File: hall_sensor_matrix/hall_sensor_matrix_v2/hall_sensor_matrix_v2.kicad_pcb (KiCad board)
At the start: 2 copper layers, 60 parts, among them J1 CTRL, J2 COL, J3 ROW, Q1 VP3203, Q2 VP3203, Q3 VP3203, Q4 VP3203, Q5 VP3203, Q6 VP3203, Q7 VP3203, Q8 VP3203, U1 74LS595, U2 74LS597, U3 74LS597

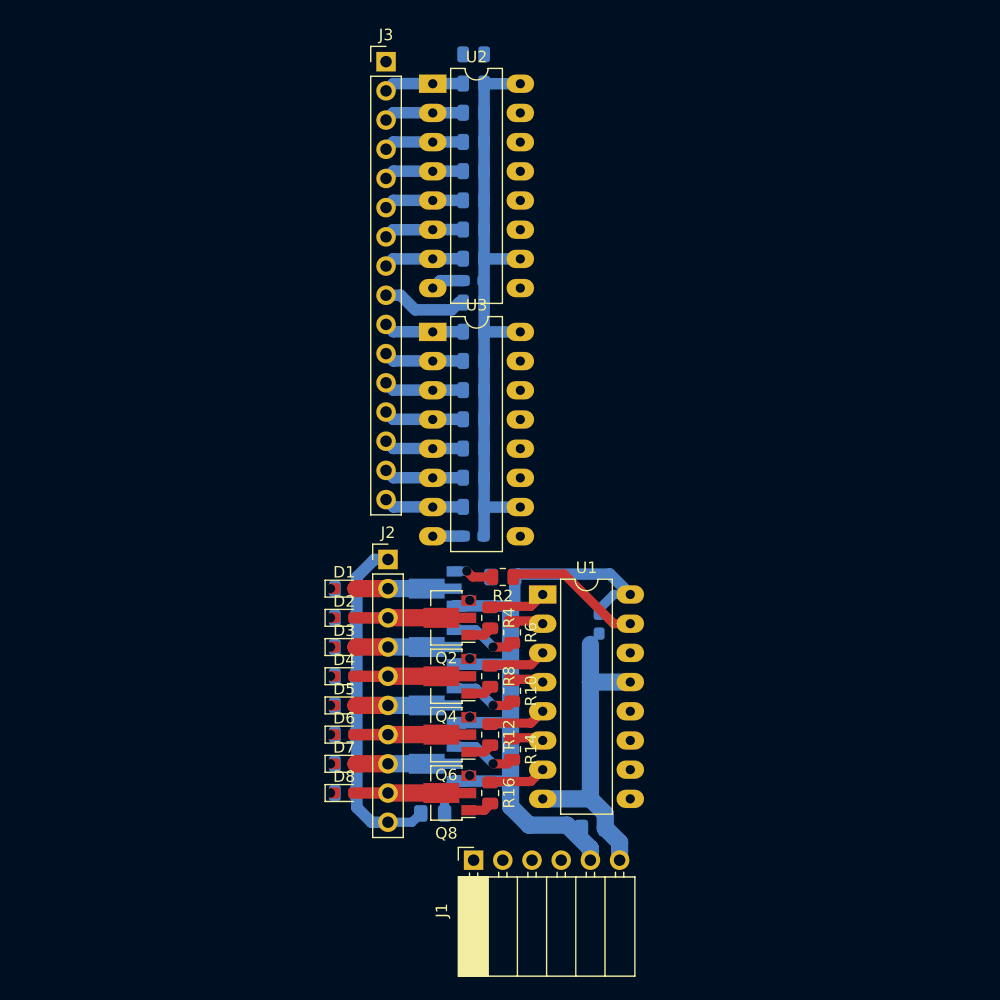
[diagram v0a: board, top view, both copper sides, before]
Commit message: added v2
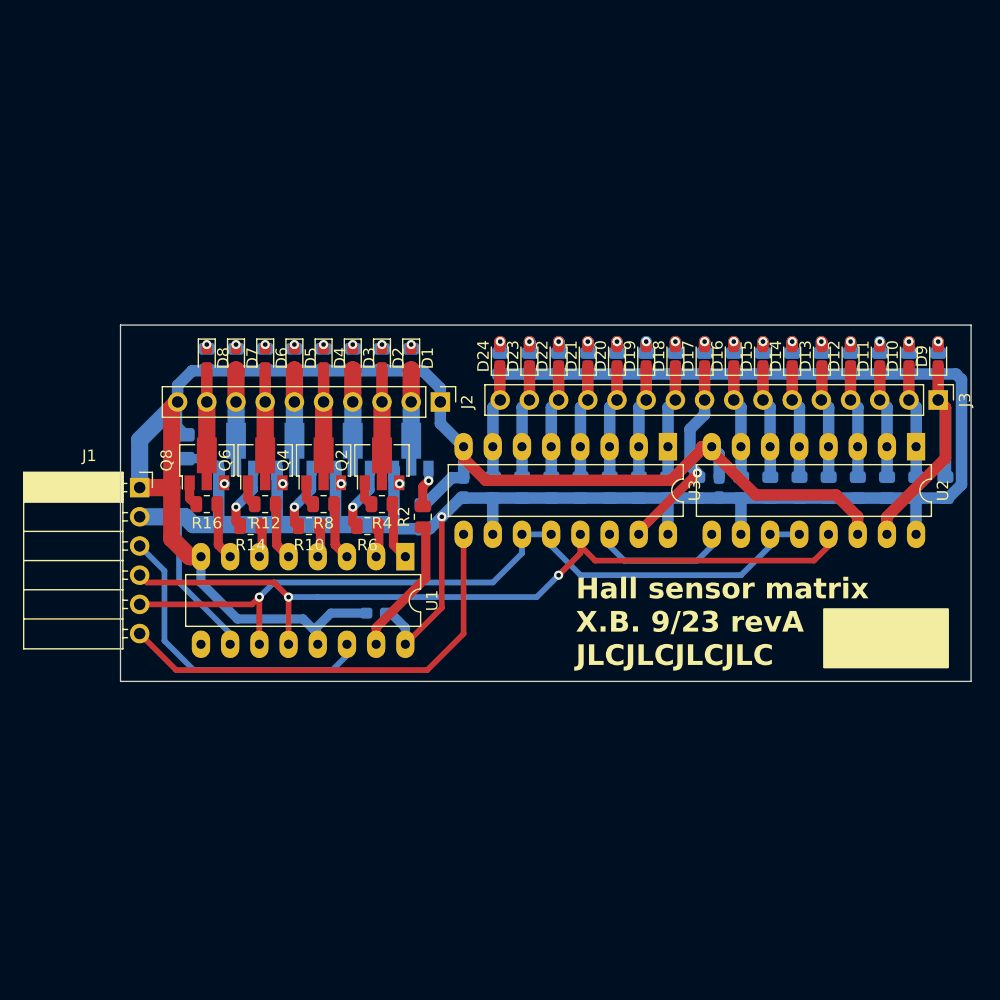
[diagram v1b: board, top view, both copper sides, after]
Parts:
- added D10: LED, LED_SMD:LED_0603_1608Metric_Pad1.05x0.95mm_HandSolder, F.Cu at (142.0, 88.5)
- added D11: LED, LED_SMD:LED_0603_1608Metric_Pad1.05x0.95mm_HandSolder, F.Cu at (139.5, 88.5)
- added D12: LED, LED_SMD:LED_0603_1608Metric_Pad1.05x0.95mm_HandSolder, F.Cu at (136.9, 88.5)
- added D13: LED, LED_SMD:LED_0603_1608Metric_Pad1.05x0.95mm_HandSolder, F.Cu at (134.4, 88.5)
- added D14: LED, LED_SMD:LED_0603_1608Metric_Pad1.05x0.95mm_HandSolder, F.Cu at (131.9, 88.5)
- added D15: LED, LED_SMD:LED_0603_1608Metric_Pad1.05x0.95mm_HandSolder, F.Cu at (129.3, 88.5)
- added D16: LED, LED_SMD:LED_0603_1608Metric_Pad1.05x0.95mm_HandSolder, F.Cu at (126.8, 88.5)
- added D17: LED, LED_SMD:LED_0603_1608Metric_Pad1.05x0.95mm_HandSolder, F.Cu at (124.2, 88.5)
- added D18: LED, LED_SMD:LED_0603_1608Metric_Pad1.05x0.95mm_HandSolder, F.Cu at (121.7, 88.5)
- added D19: LED, LED_SMD:LED_0603_1608Metric_Pad1.05x0.95mm_HandSolder, F.Cu at (119.2, 88.5)
- added D20: LED, LED_SMD:LED_0603_1608Metric_Pad1.05x0.95mm_HandSolder, F.Cu at (116.6, 88.5)
- added D21: LED, LED_SMD:LED_0603_1608Metric_Pad1.05x0.95mm_HandSolder, F.Cu at (114.1, 88.5)
- added D22: LED, LED_SMD:LED_0603_1608Metric_Pad1.05x0.95mm_HandSolder, F.Cu at (111.5, 88.5)
- added D23: LED, LED_SMD:LED_0603_1608Metric_Pad1.05x0.95mm_HandSolder, F.Cu at (109.0, 88.5)
- added D24: LED, LED_SMD:LED_0603_1608Metric_Pad1.05x0.95mm_HandSolder, F.Cu at (106.4, 88.5)
- added D9: LED, LED_SMD:LED_0603_1608Metric_Pad1.05x0.95mm_HandSolder, F.Cu at (144.6, 88.5)
- added R33: 470, Resistor_SMD:R_0805_2012Metric, B.Cu at (144.6, 89.1)
- added R34: 470, Resistor_SMD:R_0805_2012Metric, B.Cu at (142.0, 89.1)
- added R35: 470, Resistor_SMD:R_0805_2012Metric, B.Cu at (139.5, 89.1)
- added R36: 470, Resistor_SMD:R_0805_2012Metric, B.Cu at (136.9, 89.1)
- added R37: 470, Resistor_SMD:R_0805_2012Metric, B.Cu at (134.4, 89.1)
- added R38: 470, Resistor_SMD:R_0805_2012Metric, B.Cu at (131.9, 89.1)
- added R39: 470, Resistor_SMD:R_0805_2012Metric, B.Cu at (129.3, 89.1)
- added R40: 470, Resistor_SMD:R_0805_2012Metric, B.Cu at (126.8, 89.1)
- added R41: 470, Resistor_SMD:R_0805_2012Metric, B.Cu at (124.2, 89.1)
- added R42: 470, Resistor_SMD:R_0805_2012Metric, B.Cu at (121.7, 89.1)
- added R43: 470, Resistor_SMD:R_0805_2012Metric, B.Cu at (119.2, 89.1)
- added R44: 470, Resistor_SMD:R_0805_2012Metric, B.Cu at (116.6, 89.1)
- added R45: 470, Resistor_SMD:R_0805_2012Metric, B.Cu at (114.1, 89.1)
- added R46: 470, Resistor_SMD:R_0805_2012Metric, B.Cu at (111.6, 89.1)
- added R47: 470, Resistor_SMD:R_0805_2012Metric, B.Cu at (109.0, 89.1)
- added R48: 470, Resistor_SMD:R_0805_2012Metric, B.Cu at (106.5, 89.1)
- moved J3 56.3 mm to (144.6, 92.3), turned to -90 degrees
- moved R17 55.7 mm to (145.2, 99.9), turned to 90 degrees
- moved U2 52.6 mm to (142.6, 96.4), turned to -90 degrees
- moved R18 52.1 mm to (142.7, 99.9), turned to 90 degrees
- moved R19 48.6 mm to (140.1, 99.9), turned to 90 degrees
- moved C2 46.4 mm to (77.9, 101.2), turned to 90 degrees
- moved R20 45.0 mm to (137.6, 99.9), turned to 90 degrees
- moved J1 43.5 mm to (75.1, 99.9), turned to 0 degrees
- moved R21 41.4 mm to (135.0, 99.9), turned to 90 degrees
- moved D8 39.7 mm to (80.9, 88.7), turned to -90 degrees
- moved R15 39.6 mm to (80.9, 88.8), turned to -90 degrees
- moved C6 38.4 mm to (79.2, 96.4), turned to 90 degrees
- moved R22 37.8 mm to (132.5, 99.9), turned to 90 degrees
- moved D7 36.5 mm to (83.5, 88.7), turned to -90 degrees
- moved R13 36.5 mm to (83.5, 88.8), turned to -90 degrees
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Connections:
- J1 pad 1: /Dout -> GND
- J1 pad 2: /Din -> +5V
- J1 pad 3: /Latch -> /Din
- J1 pad 4: /CLK -> /Latch
- J1 pad 5: +5V -> /CLK
- J1 pad 6: GND -> /Dout
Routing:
- net GND: track 62.9 -> 136.6 mm
- net /Latch: track 0.00 -> 71.1 mm, vias 0 -> 2
- net /CLK: track 0.00 -> 69.1 mm, vias 0 -> 1
- net +5V: track 125.2 -> 193.7 mm, vias 4 -> 5
- net /Dout: track 0.00 -> 39.5 mm
- net /Din: track 0.00 -> 27.6 mm
- net /R0: track 0.00 -> 24.0 mm
- net /Dout_1: track 0.00 -> 12.0 mm
- net /R8: track 7.50 -> 17.5 mm, vias 0 -> 1
- net /R4: track 6.97 -> 9.93 mm
- net /R15: track 6.97 -> 9.92 mm
- net /R5: track 6.97 -> 9.91 mm
- net /R1: track 6.97 -> 9.91 mm
- net /R7: track 6.97 -> 9.91 mm
- net /R14: track 6.97 -> 9.91 mm
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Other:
- board outline added: 74 x 31 mm
- board text added: "Hall sensor matrix X.B. 9/23 revA JLCJLCJLCJLC"
